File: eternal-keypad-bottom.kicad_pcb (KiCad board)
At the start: 2 copper layers, 169.9 x 95.3 mm, 5 parts

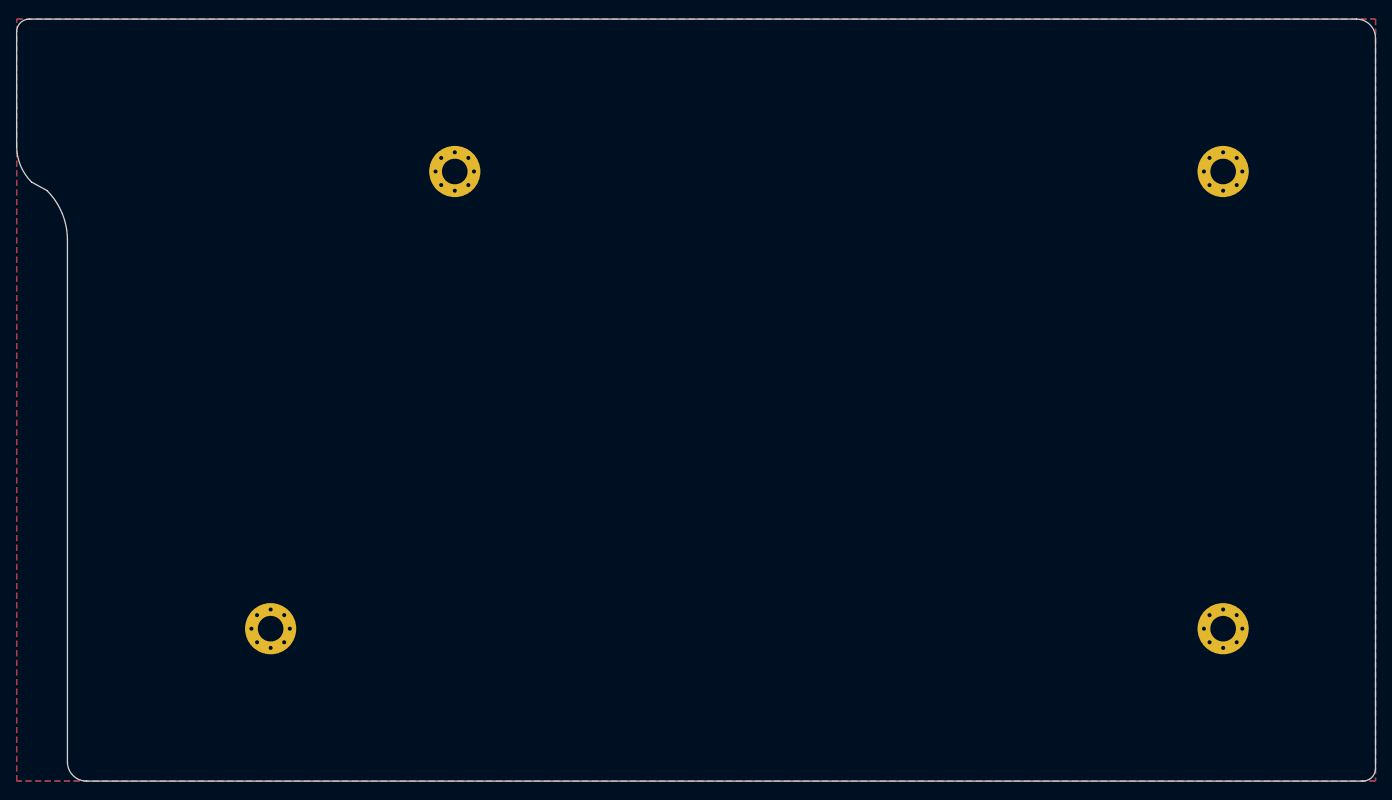
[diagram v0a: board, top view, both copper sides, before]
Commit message: Final adjustments and case patterns
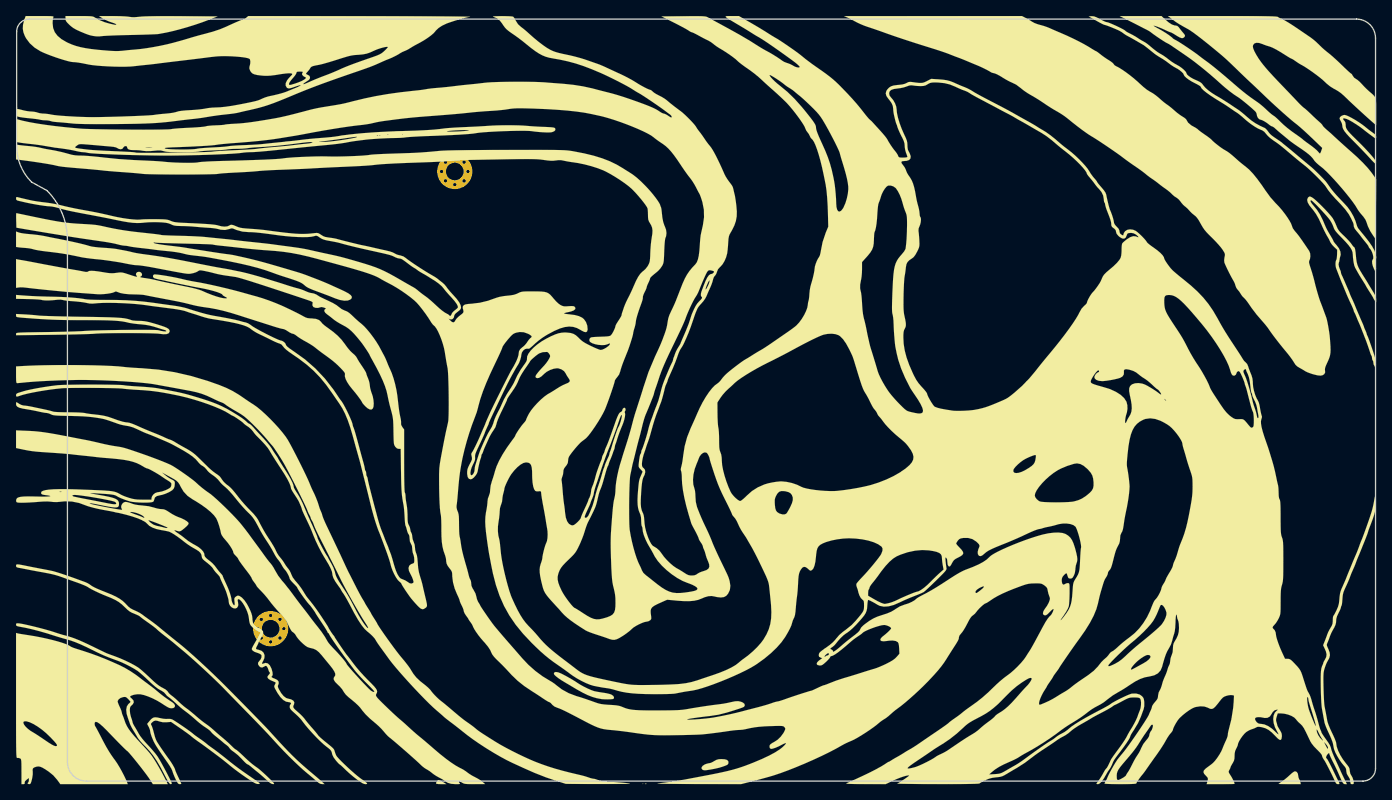
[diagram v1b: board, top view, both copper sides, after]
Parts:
- removed the REF** at (102.4, 58.7)
- removed the REF** at (79.4, 115.9)
- added G***: LOGO, Symbol:paint-swirl, B.Cu at (132.6, 87.3)
- added G***: LOGO, Symbol:paint-swirl, F.Cu at (132.6, 87.3)
- added REF**: MountingHole_4.6mm_Pad_Via, MountingHole:MountingHole_2.2mm_M2_Pad_Via, F.Cu at (102.4, 58.7)
- added REF**: MountingHole_4.6mm_Pad_Via, MountingHole:MountingHole_2.2mm_M2_Pad_Via, F.Cu at (79.4, 115.9)
- REF** (x2): value MountingHole_3.2mm_M3_Pad_Via -> MountingHole_4.6mm_Pad_Via; footprint MountingHole:MountingHole_3.2mm_M3_Pad_Via -> MountingHole:MountingHole_2.2mm_M2_Pad_Via
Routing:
- removed copper zone on B.Cu, net GND
- removed copper zone on F.Cu, net GND
